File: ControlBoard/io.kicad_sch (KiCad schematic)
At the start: 10 parts, among them U1 USBLC6-2P6

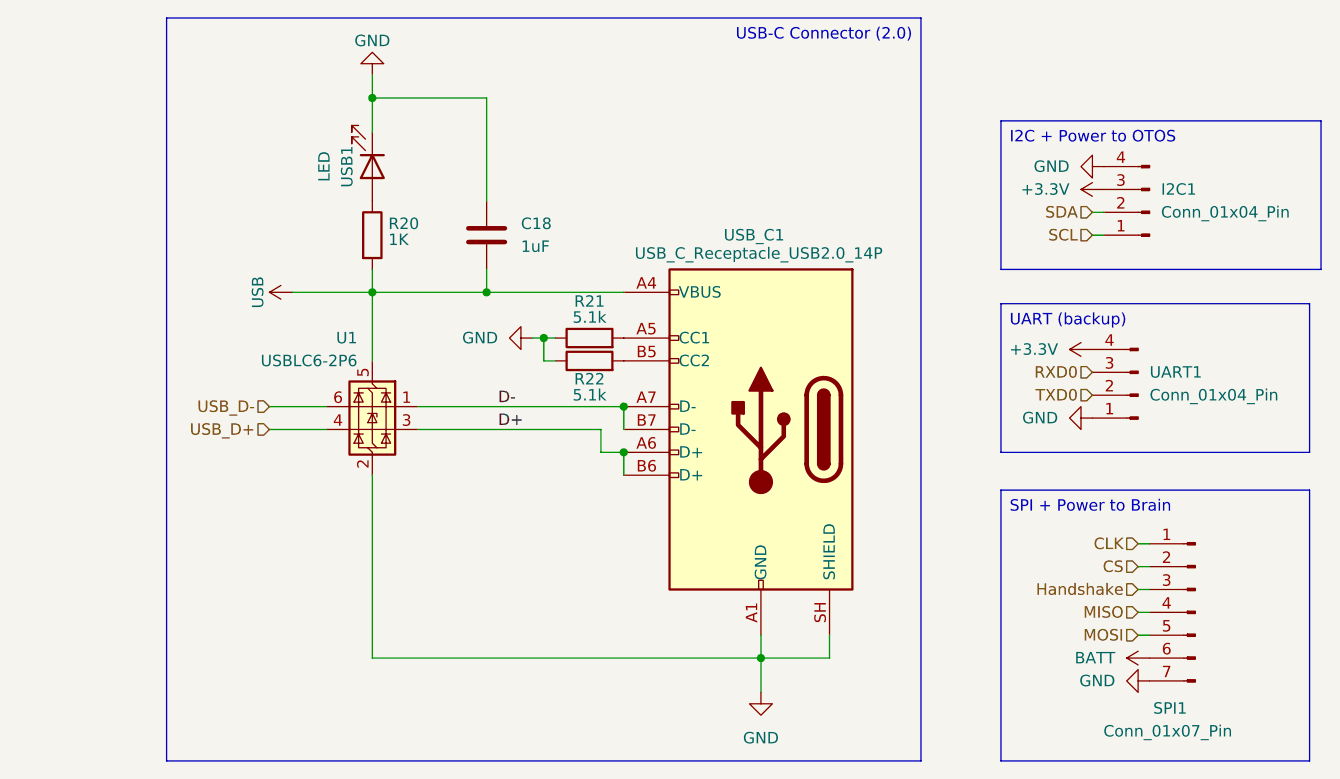
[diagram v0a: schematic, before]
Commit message: Updates to schematic by Ludo <3
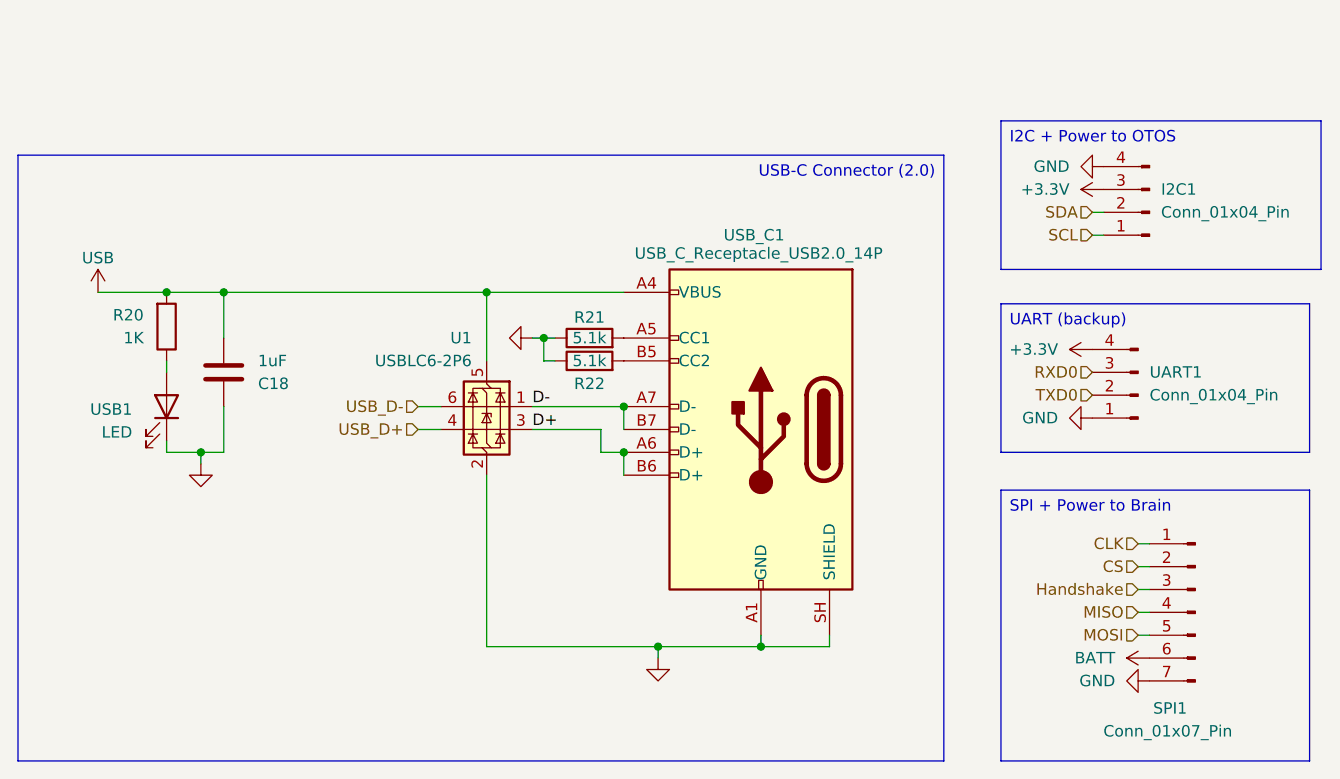
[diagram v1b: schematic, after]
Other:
- moved on the sheet: C18, R20, U1, USB1
